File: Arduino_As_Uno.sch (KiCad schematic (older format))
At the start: 8 parts, among them P1 Power, P2 Analog, P3 Digital, P4 Digital, P5 CONN_1, P6 CONN_1, P7 CONN_1, P8 CONN_1

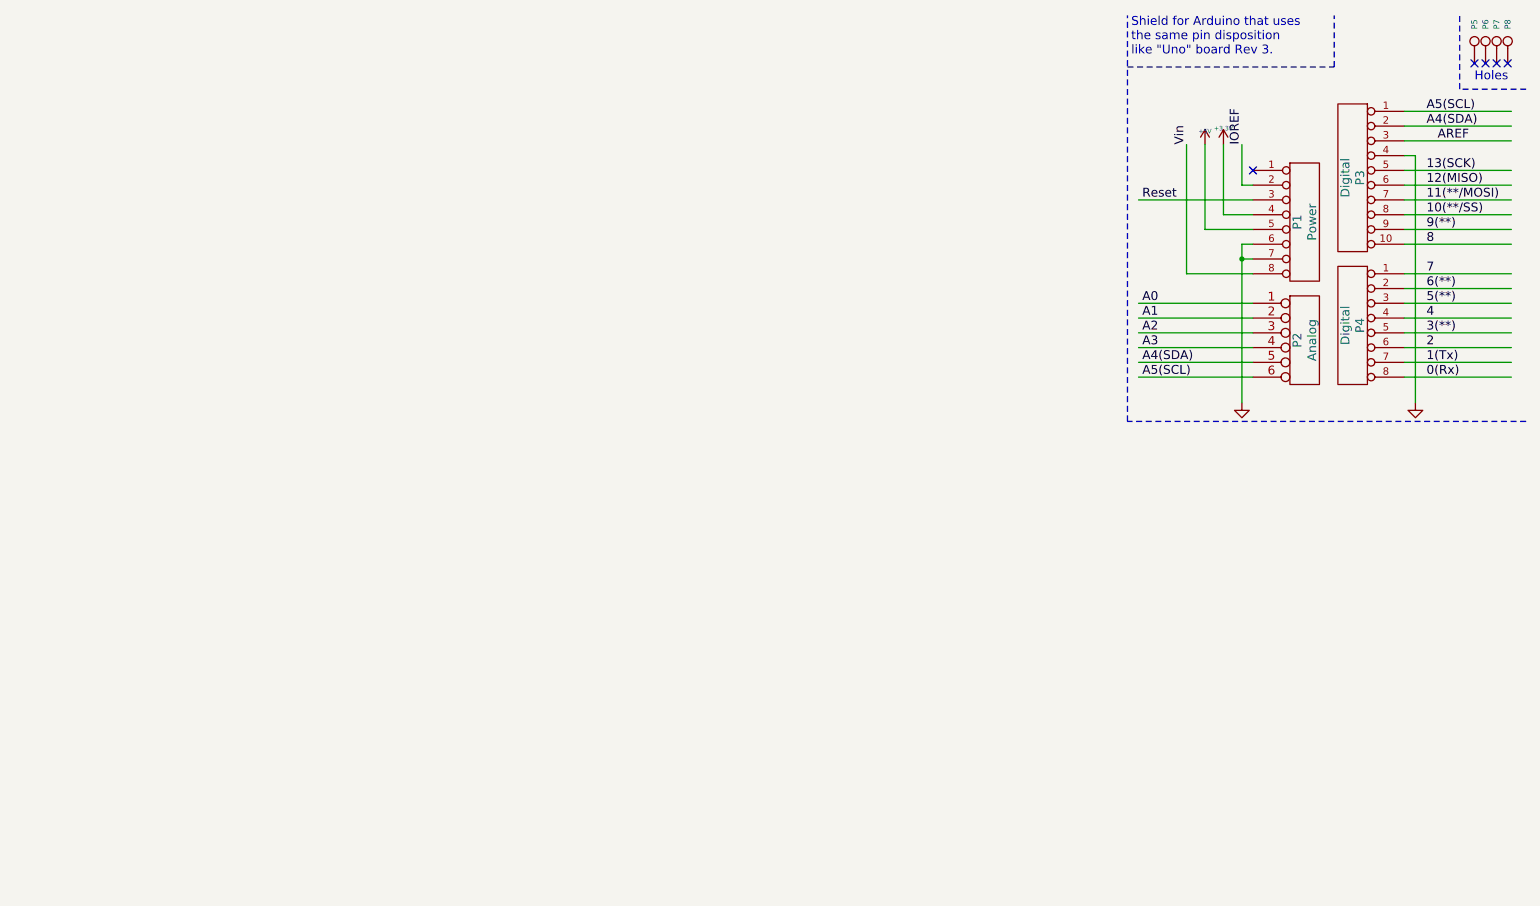
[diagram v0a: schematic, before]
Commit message: First design sent out.
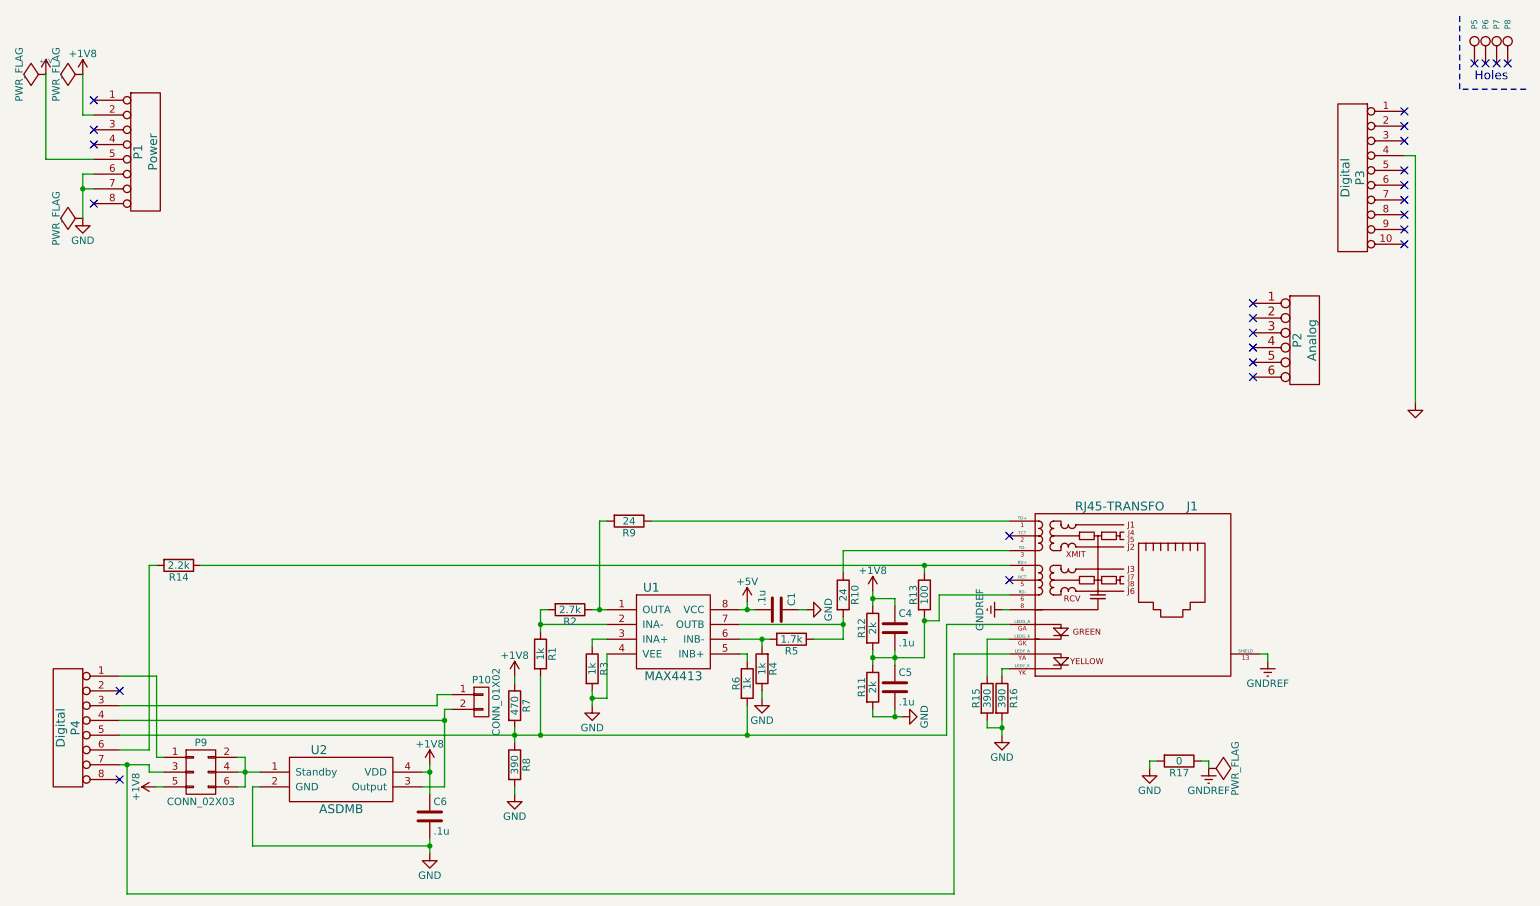
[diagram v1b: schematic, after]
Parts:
- added C1, C4, C5, C6: .1u, Capacitors_SMD:C_0805_HandSoldering, symbol C
- added J1: RJ45-TRANSFO, ga-ethernet:RJ45_TRANSFO, symbol RJ45-TRANSFO
- added P10: CONN_01X02, Pin_Headers:Pin_Header_Straight_1x02, symbol CONN_01X02
- added P9: CONN_02X03, Pin_Headers:Pin_Header_Straight_2x03, symbol CONN_02X03
- added R1, R3, R4, R6: 1k, Resistors_SMD:R_0805_HandSoldering, symbol R
- added R10, R9: 24, Resistors_SMD:R_2512_HandSoldering, symbol R
- added R11, R12: 2k, Resistors_SMD:R_0805_HandSoldering, symbol R
- added R13: 100, Resistors_SMD:R_2512_HandSoldering, symbol R
- added R14: 2.2k, Resistors_SMD:R_0805_HandSoldering, symbol R
- added R15, R16, R8: 390, Resistors_SMD:R_0805_HandSoldering, symbol R
- added R17: 0, Resistors_SMD:R_2512_HandSoldering, symbol R
- added R2: 2.7k, Resistors_SMD:R_0805_HandSoldering, symbol R
- added R5: 1.7k, Resistors_SMD:R_0805_HandSoldering, symbol R
- added R7: 470, Resistors_SMD:R_0805_HandSoldering, symbol R
- added U1: MAX4413, ga-ethernet:SOT-23-8, symbol MAX4413
- added U2: ASDMB, ga-ethernet:ASDMB, symbol ASDMB
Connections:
- net labels added: +1V8, GNDREF
- net labels removed: +3.3V, 0(Rx), 1(Tx), 10(**/SS), 11(**/MOSI), 12(MISO), 13(SCK), 2, 3(**), 4, 5(**), 6(**), 7, 8, 9(**), A0, A1, A2, A3, A4(SDA), A5(SCL), AREF, IOREF, Reset, Vin
- wire segments 37 -> 102
- no-connect marks 5 -> 27
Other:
- note removed: "Shield for Arduino that uses\nthe same pin disposition\nlike "Uno" board Rev 3."
- moved on the sheet: P1, P4
